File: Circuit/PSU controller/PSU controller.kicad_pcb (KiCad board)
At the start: 2 copper layers, 47.6 x 32.4 mm, 13 parts, among them Q1 S8050

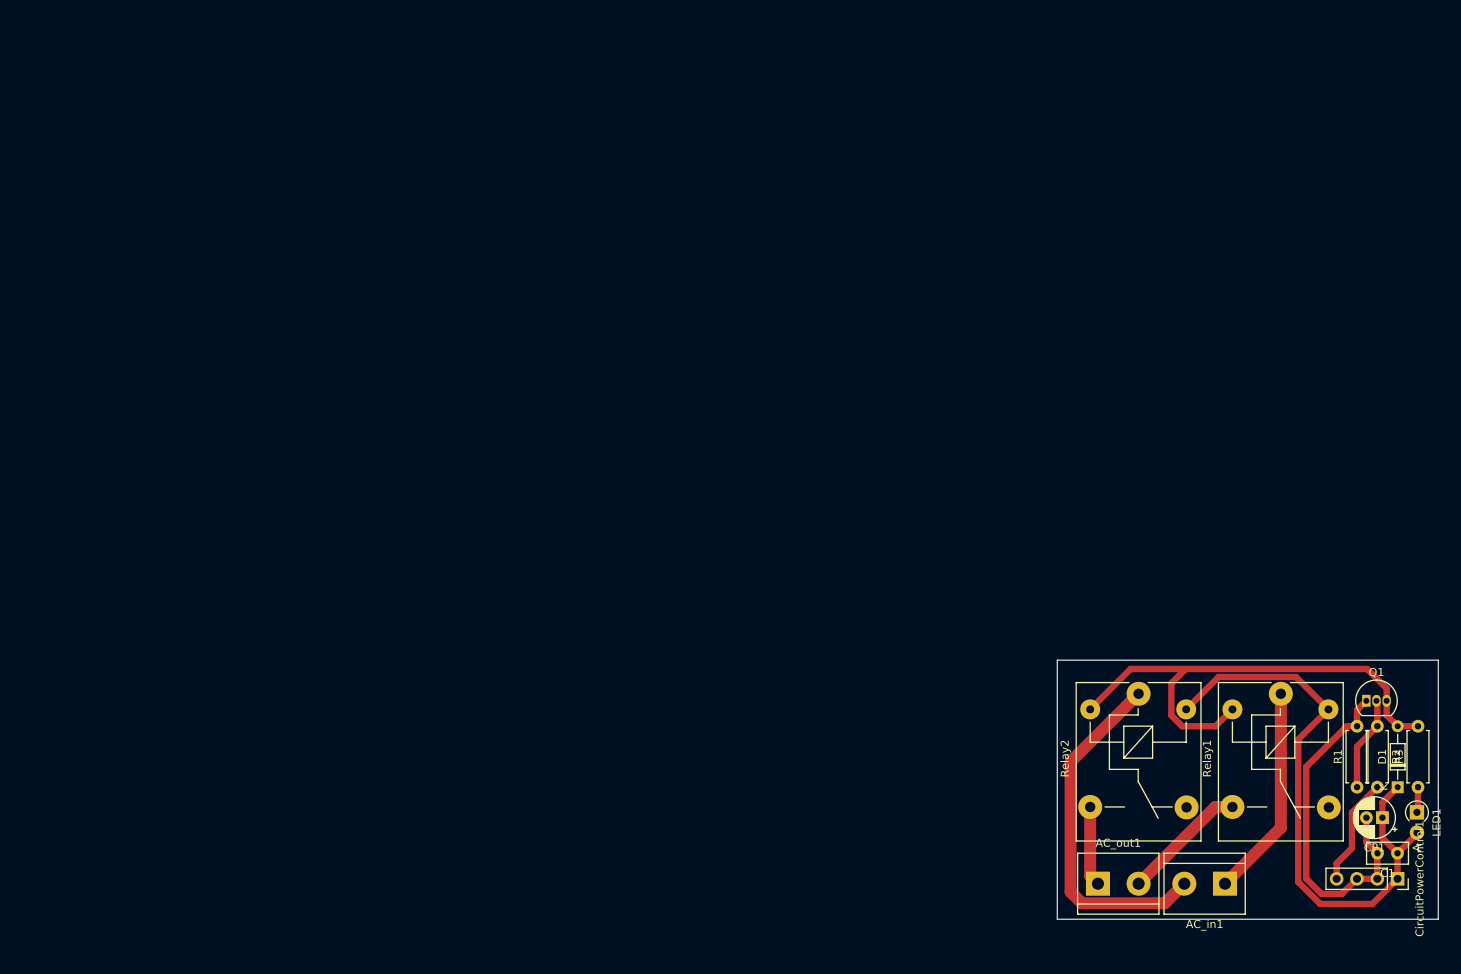
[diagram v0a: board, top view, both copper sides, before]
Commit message: all files updated after OS change for some reason
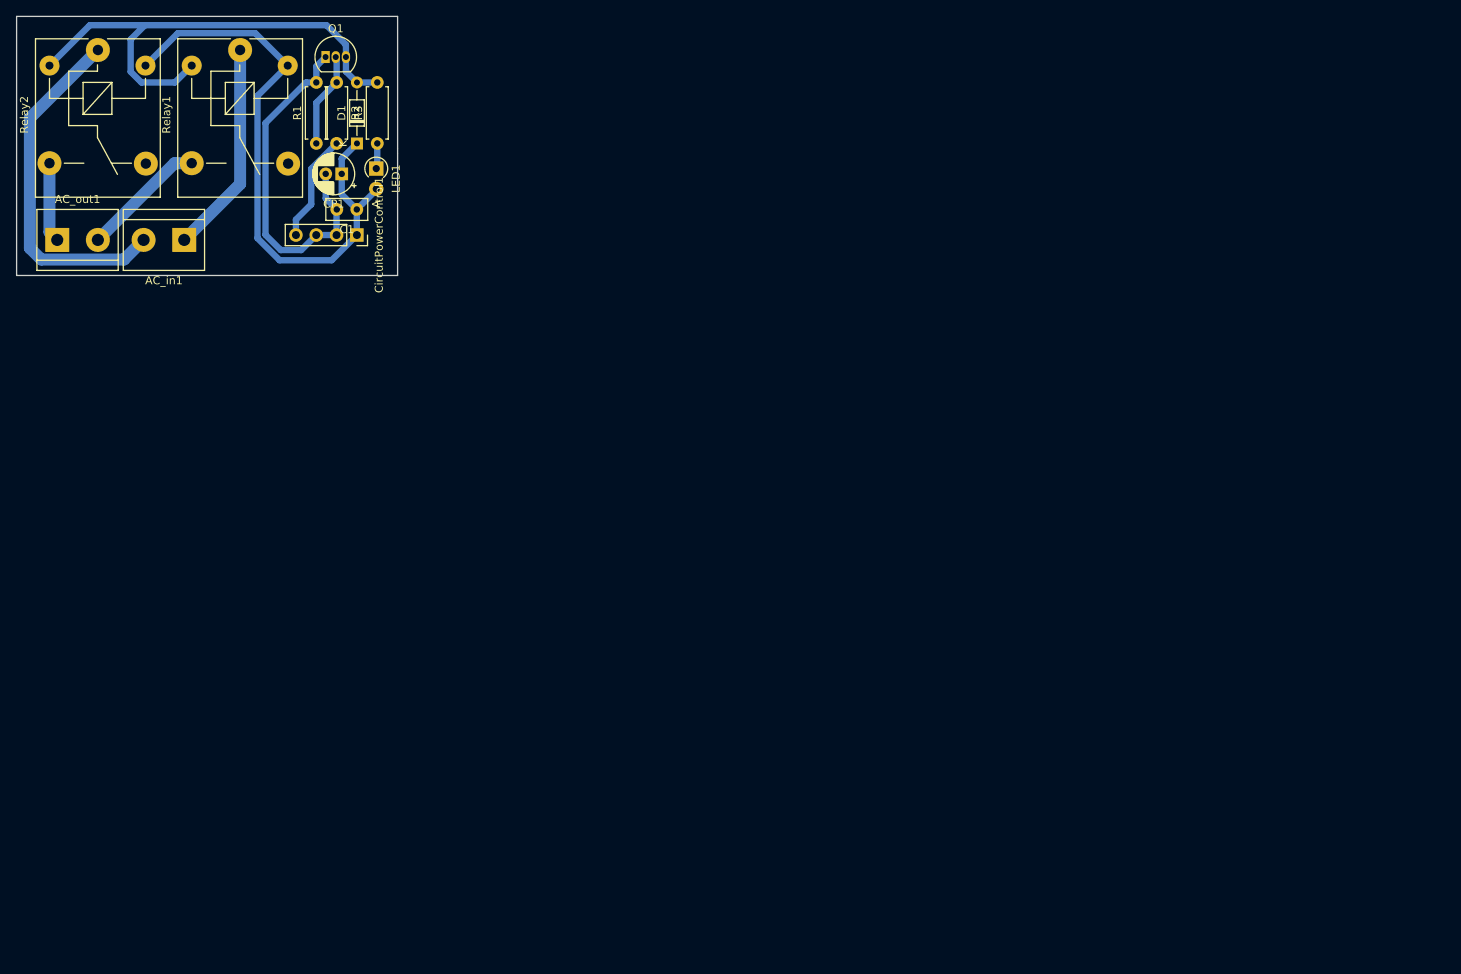
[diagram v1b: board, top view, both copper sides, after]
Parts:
- moved AC_in1 153.0 mm to (21.3, 28.2)
- moved AC_out1 153.0 mm to (5.42, 28.2)
- moved C1 153.0 mm to (42.9, 24.4)
- moved CircuitPowerControl1 153.0 mm to (42.9, 27.6)
- moved D1 153.0 mm to (42.9, 16.2)
- moved LED1 153.0 mm to (45.3, 19.3)
- moved Q1 153.0 mm to (39.0, 5.38)
- moved R1 153.0 mm to (37.8, 16.2)
- moved R2 153.0 mm to (40.3, 8.55)
- moved R3 153.0 mm to (45.4, 16.2)
- moved CP1 153.0 mm to (41.0, 20.0)
- moved Relay1 153.0 mm to (28.3, 4.50)
- moved Relay2 153.0 mm to (10.5, 4.50)

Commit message: further development in esp32-cam
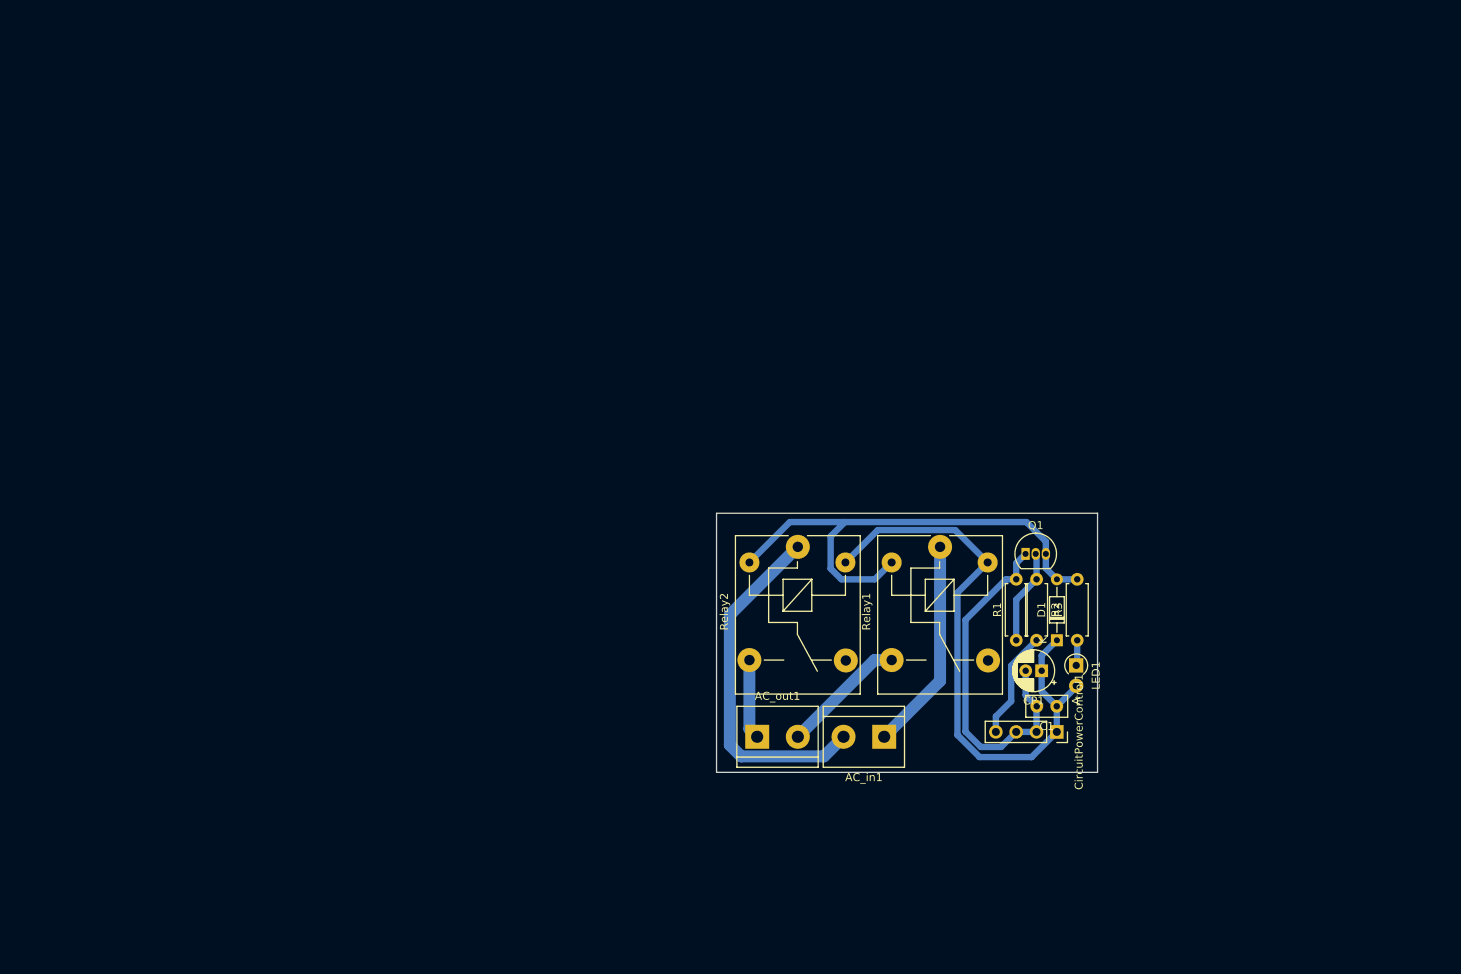
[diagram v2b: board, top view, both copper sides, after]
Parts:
- moved AC_in1 107.3 mm to (108.8, 90.3)
- moved AC_out1 107.3 mm to (92.9, 90.3)
- moved C1 107.3 mm to (130.4, 86.5)
- moved D1 107.3 mm to (130.4, 78.3)
- moved R2 107.3 mm to (127.8, 70.7)
- moved R3 107.3 mm to (132.9, 78.3)
- moved CP1 107.3 mm to (128.5, 82.1)
- moved CircuitPowerControl1 107.3 mm to (130.4, 89.7)
- moved LED1 107.3 mm to (132.8, 81.4)
- moved Q1 107.3 mm to (126.5, 67.5)
- moved R1 107.3 mm to (125.3, 78.3)
- moved Relay1 107.3 mm to (115.8, 66.6)
- moved Relay2 107.3 mm to (98.0, 66.6)
